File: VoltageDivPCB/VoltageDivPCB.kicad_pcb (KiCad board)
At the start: 2 copper layers, 10.2 x 15.2 mm, 7 parts, among them J1 Conn_01x04

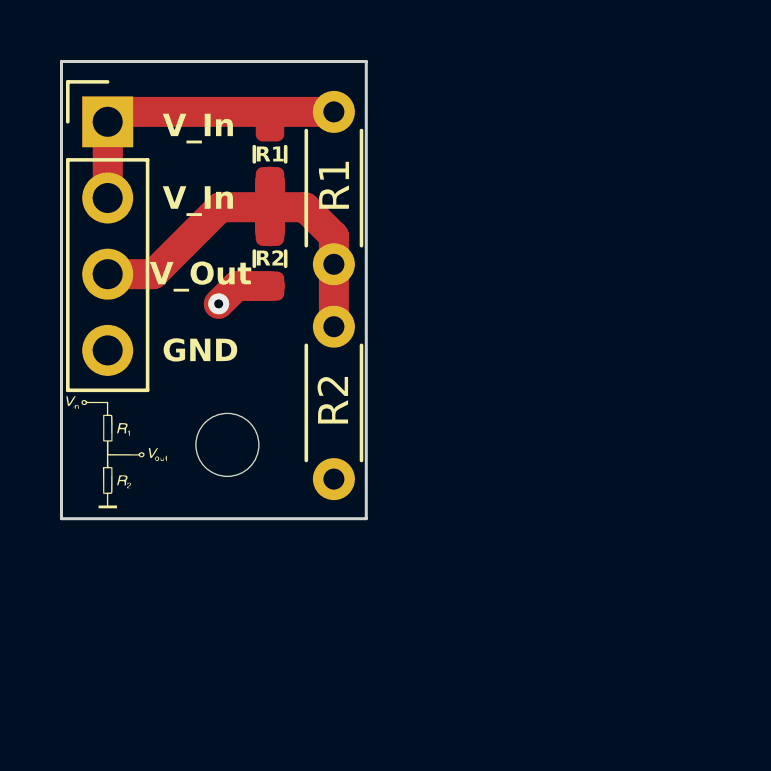
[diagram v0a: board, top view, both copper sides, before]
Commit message: Lab jack work
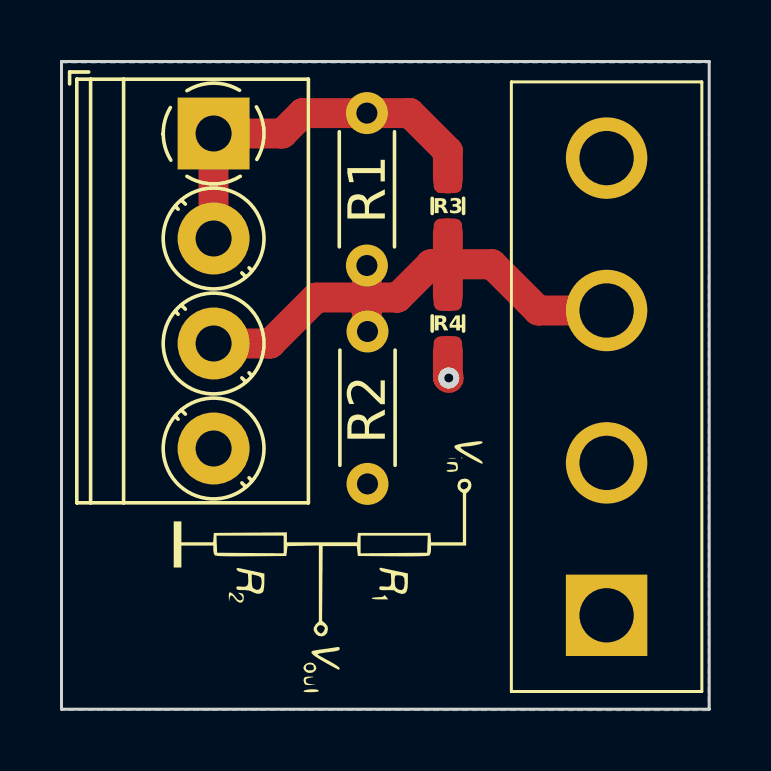
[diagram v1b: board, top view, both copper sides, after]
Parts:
- removed H1: MountingHole_Pad, MountingHole:MountingHole_2.1mm
- removed the R1 at (34.5, 27.1)
- removed the R1 at (32.4, 28.5)
- removed the R2 at (32.4, 32.0)
- removed the R2 at (34.5, 34.2)
- added J2: Screw_Terminal_01x04, TerminalBlock_Phoenix:TerminalBlock_Phoenix_PT-1,5-4-3.5-H_1x04_P3.50mm_Horizontal, F.Cu at (30.5, 27.8)
- added R1: Solderable, Resistor_THT:R_Axial_DIN0204_L3.6mm_D1.6mm_P5.08mm_Horizontal, F.Cu at (35.6, 27.1)
- added R2: Solderable, Resistor_THT:R_Axial_DIN0204_L3.6mm_D1.6mm_P5.08mm_Horizontal, F.Cu at (35.6, 34.4)
- added R3: Solderable, Resistor_SMD:R_0603_1608Metric_Pad0.98x0.95mm_HandSolder, F.Cu at (38.3, 30.2)
- added R4: Solderable, Resistor_SMD:R_0603_1608Metric_Pad0.98x0.95mm_HandSolder, F.Cu at (38.3, 34.1)
- J1: value Conn_01x04 -> FWS-04-02-T-S-RA; footprint Connector_PinHeader_2.54mm:PinHeader_1x04_P2.54mm_Vertical -> FWS-04-02-T-S-RA:FWS0402TSRA
- moved J1 23.4 mm to (43.6, 43.9), turned to -90 degrees
- moved G*** 7.93 mm to (34.2, 42.3), turned to -90 degrees
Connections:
- J1 pad 1: V In -> unconnected-(J1-Pad1)
- J1 pad 2: V In -> GND
- J1 pad 4: GND -> unconnected-(J1-Pad4)
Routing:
- net V Out: track 13.5 -> 19.1 mm
- net V In: track 10.2 -> 13.0 mm
- net GND: track 1.96 -> 0.92 mm
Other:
- board size 10.2 x 15.2 mm -> 21.6 x 21.6 mm
- board text added: "SMD IS 0603"
- board text added: "V_IN"
- board text added: "V_OUT"
- board text removed: "SMD IS 0603 PAD"
- board text removed: "V_In"
- board text removed: "V_O=V_I*(R2/(R1+R2))"
- board text removed: "V_Out"
